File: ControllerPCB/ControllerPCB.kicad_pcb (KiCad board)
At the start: 4 copper layers, 185 parts, among them J101 2x4 Pickup Conn, J102 1x4 String Output Conn, J103 Conn_01x03_Pin, J104 Conn_01x03_Pin, J105 Conn_01x03_Pin, J106 Conn_01x03_Pin, J107 USB_B_Micro, J108 10-pin Debug Conn, J109 Conn_01x03_Pin, J201 9V Humbucker OUT, J202 9V IN, J301 MIDI Out Conn, J501 2x20 Conn_1, J502 2x20 Conn_2, U101 STM32F439ZIT6, U201 ADP3336ARMZ, U301 74LVC1G17, Y101 16MHz

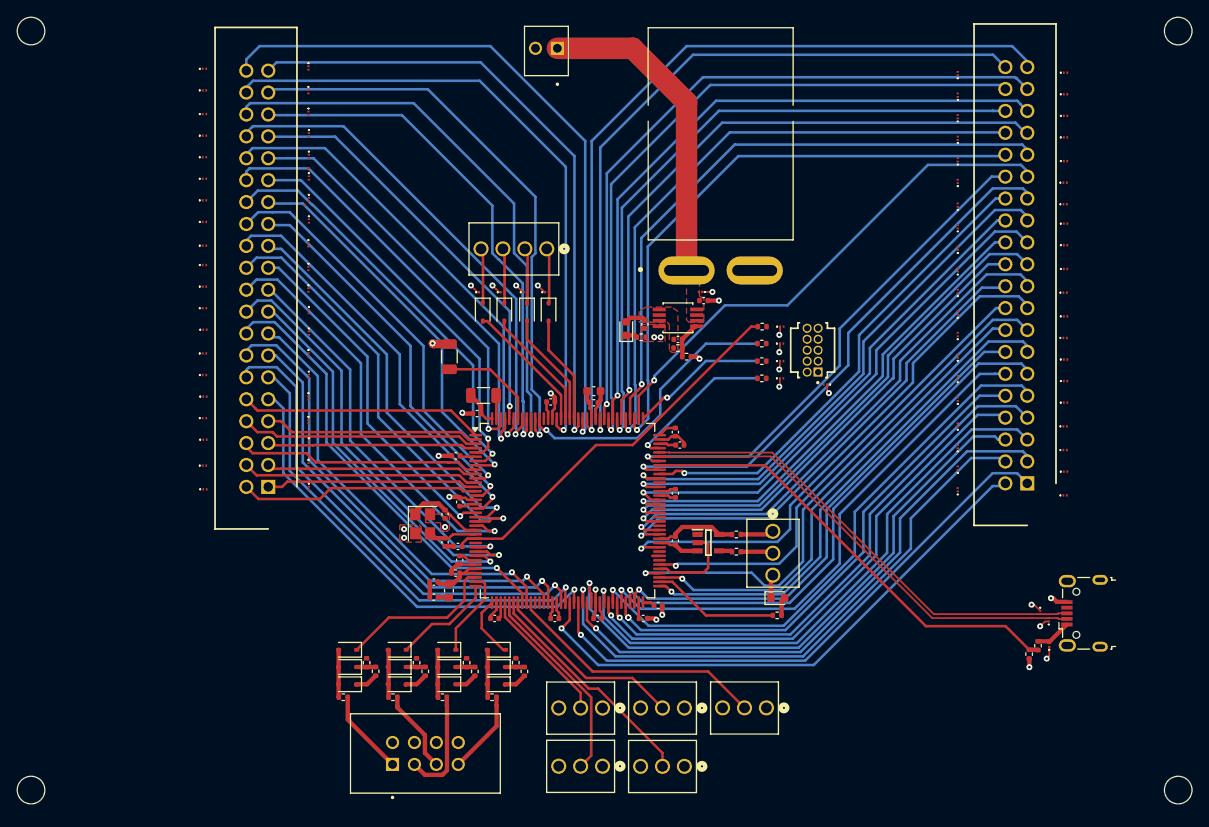
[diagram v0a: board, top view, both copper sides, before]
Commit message: rev 1.0
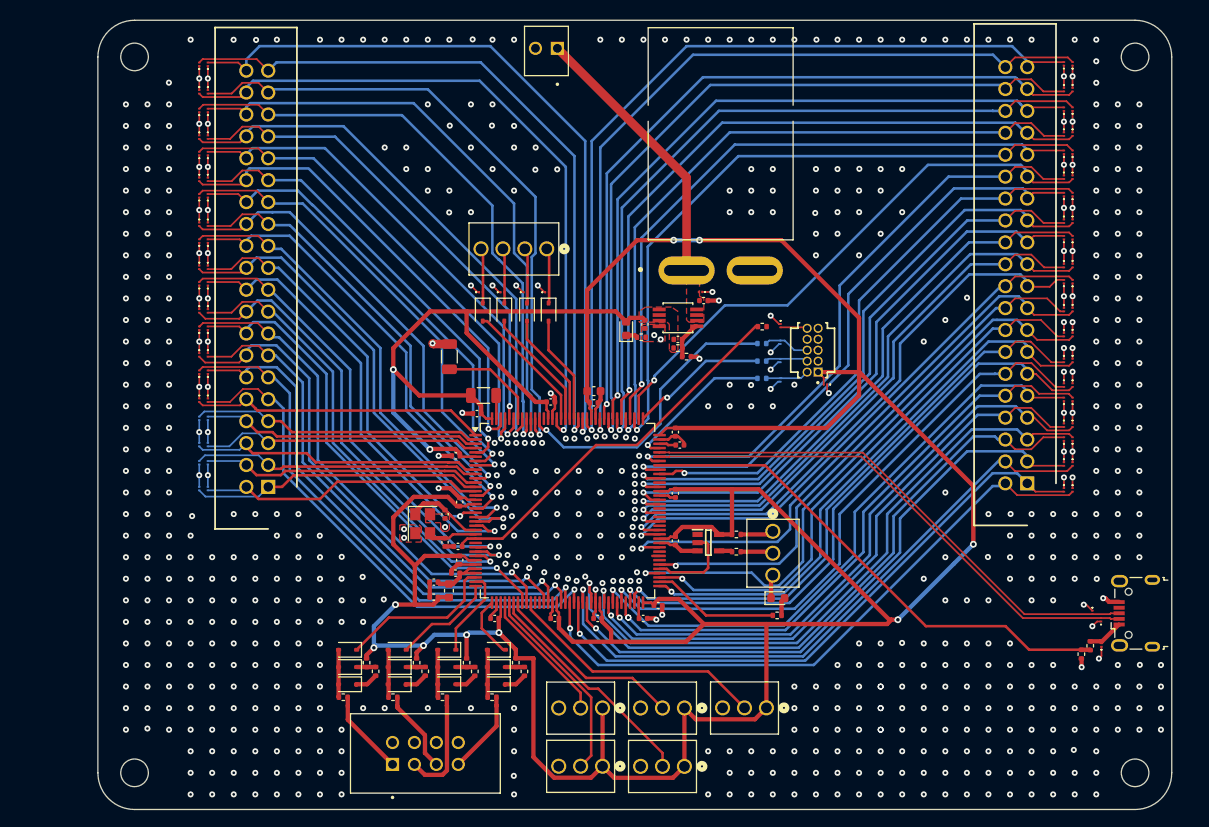
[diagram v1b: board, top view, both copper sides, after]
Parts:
- D104, D107, D111, D513, D514, D515, D516, D517, D518, D519, D520, R104, R105, R106: moved to B.Cu
- moved D579 104.1 mm to (194.8, 86.0), turned to -90 degrees
- moved D573 102.9 mm to (194.8, 83.1), turned to 90 degrees
- moved D571 102.8 mm to (194.8, 80.9), turned to -90 degrees
- moved D503 102.8 mm to (93.5, 91.3), turned to -90 degrees
- moved D502 102.7 mm to (93.5, 88.5), turned to 90 degrees
- moved D577 102.5 mm to (193.8, 86.0), turned to -90 degrees
- moved D575 102.4 mm to (193.8, 83.1), turned to 90 degrees
- moved D501 102.3 mm to (94.5, 88.5), turned to 90 degrees
- moved D563 101.9 mm to (194.8, 75.8), turned to -90 degrees
- moved D565 101.9 mm to (194.8, 78.1), turned to 90 degrees
- moved D507 101.7 mm to (93.5, 96.4), turned to -90 degrees
- moved D506 101.7 mm to (93.5, 93.6), turned to 90 degrees
- moved D567 101.5 mm to (193.8, 78.1), turned to 90 degrees
- moved D569 101.4 mm to (193.8, 80.9), turned to -90 degrees
- moved D557 101.4 mm to (194.8, 73.2), turned to 90 degrees
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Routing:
- net +3.3V: track 39.9 -> 458.8 mm, vias 0 -> 11
- net GND: track 74.8 -> 185.1 mm, vias 30 -> 680
- net input_5: track 0.00 -> 32.6 mm
- net input_43: track 91.8 -> 71.9 mm
- net input_68: track 56.0 -> 66.8 mm
- net input_70: track 59.0 -> 69.8 mm
- net input_64: track 57.9 -> 68.0 mm
- net input_66: track 58.4 -> 68.2 mm
- net input_1: track 24.5 -> 33.9 mm
- net input_23: track 45.9 -> 55.0 mm
- net input_62: track 57.5 -> 66.5 mm
- net input_3: track 24.5 -> 33.4 mm
- net input_50: track 60.2 -> 69.0 mm
- net input_39: track 73.6 -> 82.4 mm
- net input_27: track 45.8 -> 54.5 mm
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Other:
- board outline added: 124.5 x 91.5 mm
